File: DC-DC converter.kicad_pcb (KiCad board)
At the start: 2 copper layers, 55 x 29.5 mm, 19 parts, among them J1 Screw_Terminal_01x02, J2 Screw_Terminal_01x02, U1 LMR33630BDDA

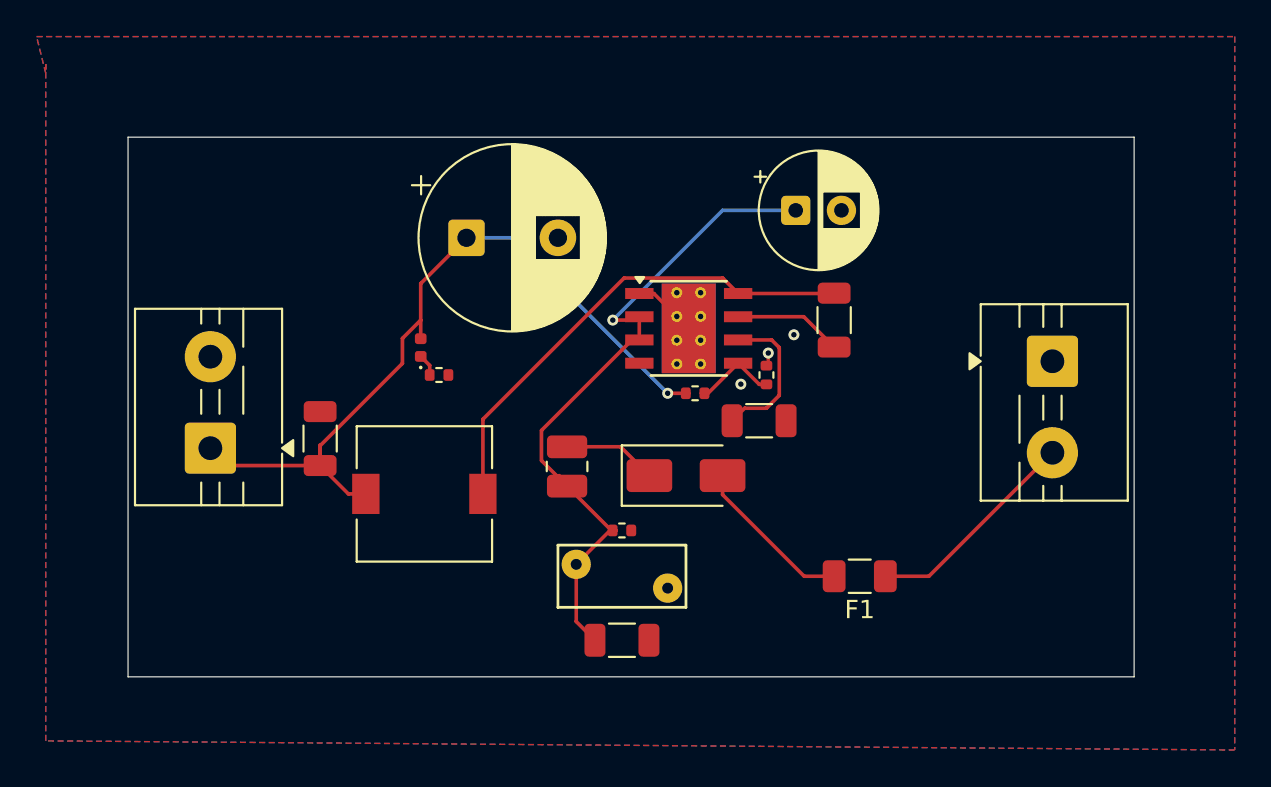
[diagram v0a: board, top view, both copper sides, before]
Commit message: submitting
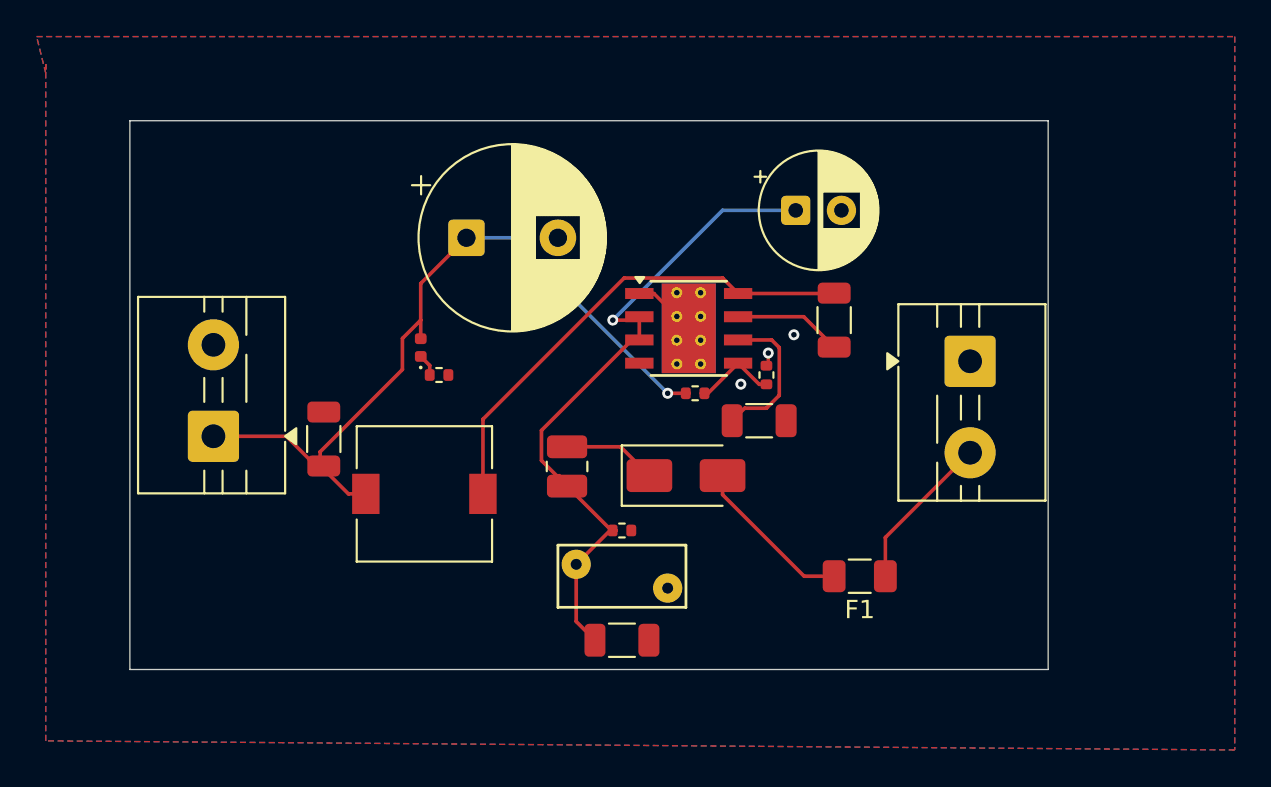
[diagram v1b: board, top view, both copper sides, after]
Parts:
- moved J1 4.50 mm to (221.0, 72.8)
- moved J2 0.67 mm to (179.7, 76.8)
- moved C3 0.20 mm to (185.7, 77.0)
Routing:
- net Net-(J1-Pin_2): track 11.9 -> 8.67 mm
- net +5V: track 43.1 -> 42.1 mm
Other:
- board size 55 x 29.5 mm -> 50.2 x 30 mm
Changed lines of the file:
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@@
 	(footprint "TerminalBlock:TerminalBlock_MaiXu_MX126-5.0-02P_1x02_P5.00mm"
 		(layer "F.Cu")
-		(at 225.5325 72.75 -90)
+		(at 221.0325 72.75 -90)
 		(descr "terminal block MaiXu MX126-5.0-02P, 2 pins, pitch 5mm, size 10.5x7.8mm, drill diameter 1.3mm, pad diameter 2.8mm, https://www.lcsc.com/datasheet/lcsc_datasheet_2309150913_MAX-MX126-5-0-03P-GN01-Cu-S-A_C5188435.pdf, script-generated using https://gitlab.com/kicad/libraries/kicad-footprint-generator/-/tree/master/scripts/TerminalBlock_MaiXu")
 		(tags "THT terminal block MaiXu MX126-5.0-02P pitch 5mm size 10.5x7.8mm drill 1.3mm pad 2.8mm")
@@
 	(footprint "Capacitor_SMD:C_1206_3216Metric"
 		(layer "F.Cu")
-		(at 185.5 76.975 90)
+		(at 185.7 77 90)
 		(descr "Capacitor SMD 1206 (3216 Metric), square (rectangular) end terminal, IPC-7351 nominal, (Body size source: IPC-SM-782 page 76, https://www.pcb-3d.com/wordpress/wp-content/uploads/ipc-sm-782a_amendment_1_and_2.pdf), generated with kicad-footprint-generator")
 		(tags "capacitor")
@@
 	(footprint "TerminalBlock:TerminalBlock_MaiXu_MX126-5.0-02P_1x02_P5.00mm"
 		(layer "F.Cu")
-		(at 179.5 77.5 90)
+		(at 179.6675 76.85 90)
 		(descr "terminal block MaiXu MX126-5.0-02P, 2 pins, pitch 5mm, size 10.5x7.8mm, drill diameter 1.3mm, pad diameter 2.8mm, https://www.lcsc.com/datasheet/lcsc_datasheet_2309150913_MAX-MX126-5-0-03P-GN01-Cu-S-A_C5188435.pdf, script-generated using https://gitlab.com/kicad/libraries/kicad-footprint-generator/-/tree/master/scripts/TerminalBlock_MaiXu")
 		(tags "THT terminal block MaiXu MX126-5.0-02P pitch 5mm size 10.5x7.8mm drill 1.3mm pad 2.8mm")
@@
 	)
 	(gr_rect
-		(start 175 60.5)
-		(end 230 90)
+		(start 175.1 59.6)
+		(end 225.3 89.6)
 		(stroke
 			(width 0.05)
@@
 	)
 	(segment
-		(start 187.05 80)
-		(end 185.5 78.45)
-		(width 0.2)
-		(layer "F.Cu")
-		(net 3)
-	)
-	(segment
-		(start 185.5 77.366544)
-		(end 190 72.866544)
+		(start 185.25 78.45)
+		(end 183.65 76.85)
 		(width 0.2)
 		(layer "F.Cu")
@@
 	)
 	(segment
-		(start 185.5 78.45)
-		(end 180.45 78.45)
+		(start 187.05 80)
+		(end 185.5 78.45)
 		(width 0.2)
 		(layer "F.Cu")
@@
 	)
 	(segment
-		(start 185.5 78.45)
-		(end 185.5 77.366544)
+		(start 191 68.5)
+		(end 193.5 66)
 		(width 0.2)
 		(layer "F.Cu")
@@
 	)
 	(segment
-		(start 191 68.5)
-		(end 193.5 66)
+		(start 183.65 76.85)
+		(end 179.6675 76.85)
 		(width 0.2)
 		(layer "F.Cu")
@@
 	)
 	(segment
-		(start 180.45 78.45)
-		(end 179.5 77.5)
+		(start 190 73.2)
+		(end 190 71.5)
 		(width 0.2)
 		(layer "F.Cu")
@@
 	)
 	(segment
-		(start 190 72.866544)
-		(end 190 71.5)
+		(start 190 71.5)
+		(end 191 70.5)
+		(width 0.2)
+		(layer "F.Cu")
+		(net 3)
+	)
+	(segment
+		(start 185.5 77.7)
+		(end 190 73.2)
 		(width 0.2)
 		(layer "F.Cu")
@@
 	)
 	(segment
-		(start 190 71.5)
-		(end 191 70.5)
+		(start 185.5 78.45)
+		(end 185.25 78.45)
 		(width 0.2)
 		(layer "F.Cu")
@@
 	(segment
 		(start 185.5 78.45)
-		(end 185.5 77.325001)
+		(end 185.5 77.7)
 		(width 0.2)
 		(layer "F.Cu")
@@
 	)
 	(segment
-		(start 216.4 84.5)
-		(end 218.7825 84.5)
+		(start 216.4 82.3825)
+		(end 221.0325 77.75)
 		(width 0.2)
 		(layer "F.Cu")
@@
 	)
 	(segment
-		(start 225.5325 77.75)
-		(end 218.7825 84.5)
+		(start 216.4 84.5)
+		(end 216.4 82.3825)
 		(width 0.2)
 		(layer "F.Cu")
